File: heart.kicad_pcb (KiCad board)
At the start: 2 copper layers, 94 x 78.7 mm, 20 parts, among them J1 Positive, J2 Negative, J3 Conn_01x19_Female, J4 Conn_01x19_Female, P1 USB_C_Plug_USB2.0, SW1 SW_DIP_x01, U1 BMD101, U2 TP4054, U3 RS3236, U5 RS8051

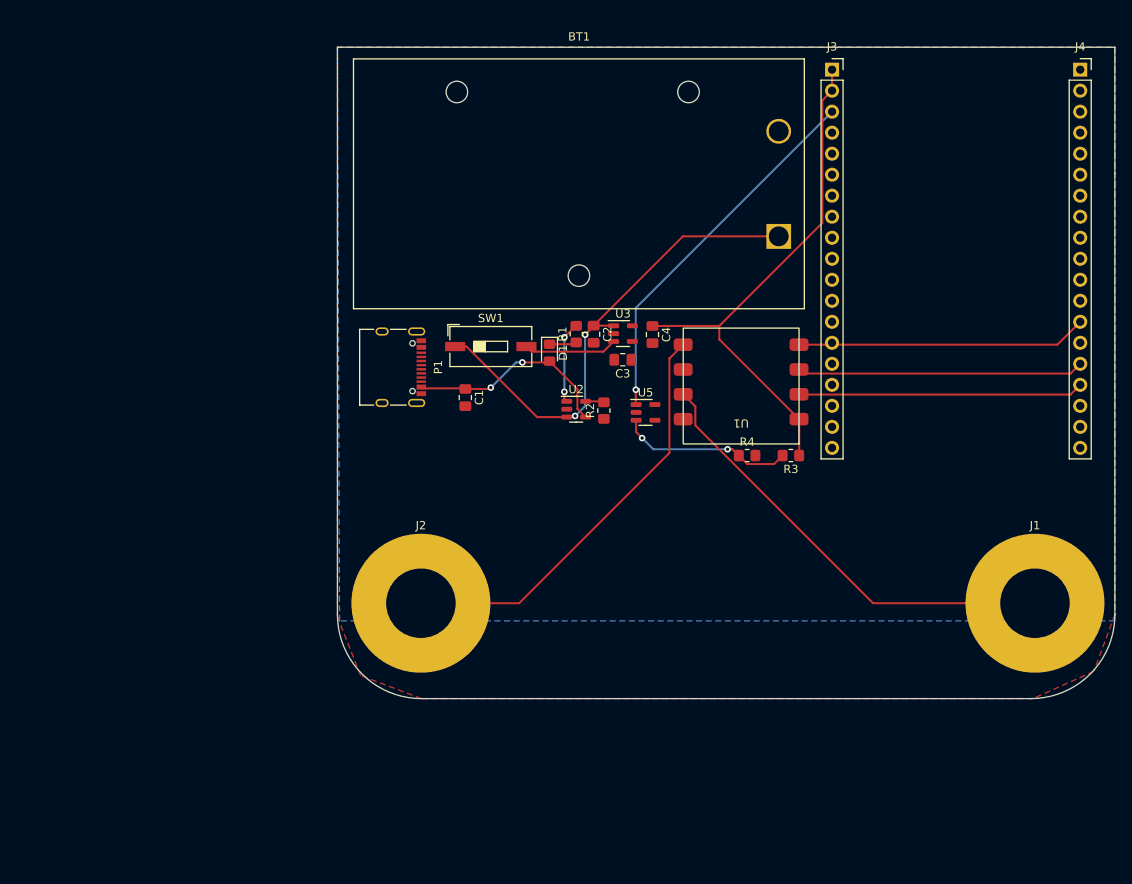
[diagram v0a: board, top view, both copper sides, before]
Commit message: 最终投板
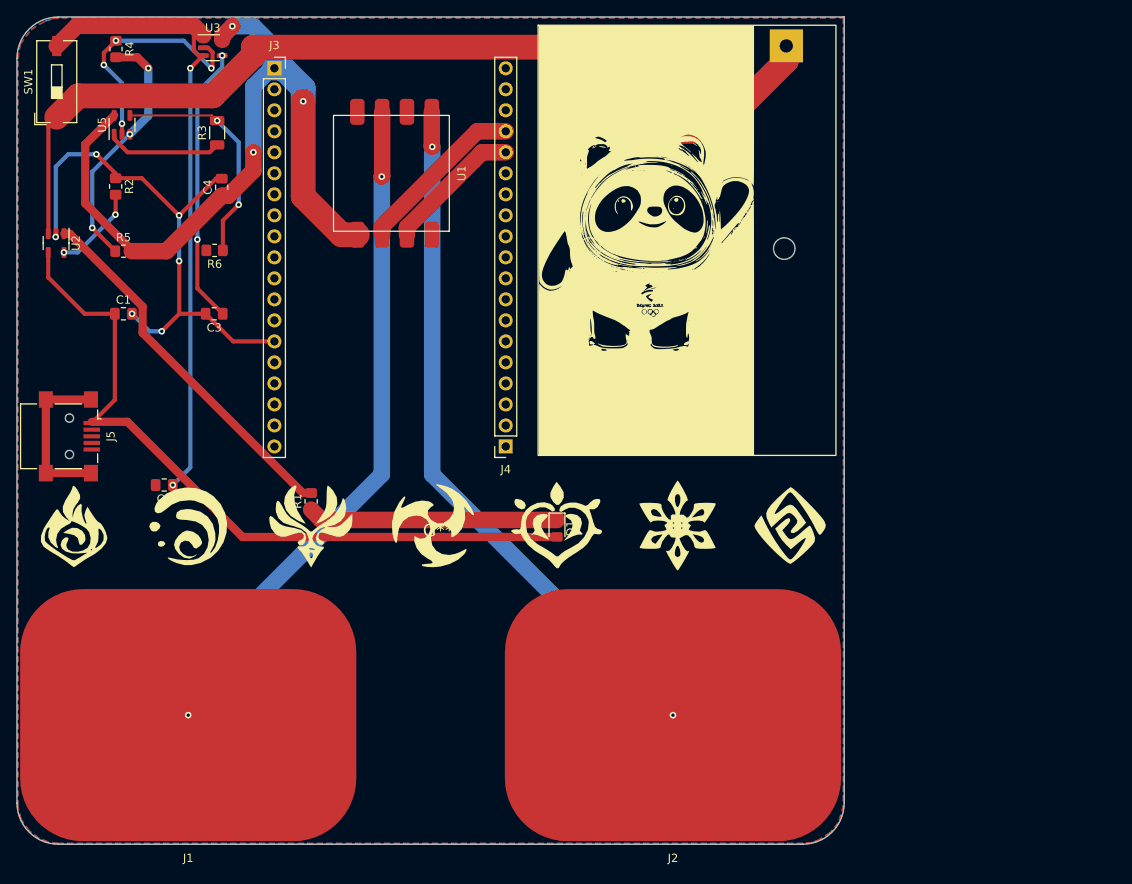
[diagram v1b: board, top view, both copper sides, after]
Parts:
- removed P1: USB_C_Plug_USB2.0, Connector_USB:USB_C_Receptacle_XKB_U262-16XN-4BVC11
- added G***: LOGO, My_Print:ys, F.Cu at (91.4, 132.1)
- added G***: LOGO, My_Print:bdd, F.Cu at (116.1, 97.0)
- added G***: LOGO, My_Print:SL_100x100, B.Cu at (89.8, 120.2)
- added J5: USB_B_Mini, Connector_USB:USB_Mini-B_Lumberg_2486_01_Horizontal, F.Cu at (46.3, 120.7)
- added R5: 30 k, Resistor_SMD:R_0805_2012Metric_Pad1.20x1.40mm_HandSolder, F.Cu at (52.9, 98.3)
- added R6: 10 k, Resistor_SMD:R_0805_2012Metric_Pad1.20x1.40mm_HandSolder, F.Cu at (63.9, 98.2)
- BT1: footprint Battery:BatteryHolder_Eagle_12BH611-GR -> My_Print:battary
- J1, J2: footprint MountingHole:MountingHole_8.4mm_M8_Pad -> My_Print:Square_Pad_40mm*30mm
- R3: footprint Resistor_SMD:R_0805_2012Metric_Pad1.20x1.40mm_HandSolder -> Resistor_SMD:R_1206_3216Metric
- R4: value 1K -> 10 k
- U1: footprint Package_TO_SOT_SMD:BMD101 -> My_Print:BMD101
- moved J1 107.0 mm to (60.7, 172.2)
- moved R4 90.8 mm to (52.0, 73.9), turned to -90 degrees
- moved J4 83.1 mm to (99.1, 121.9), turned to 180 degrees
- moved R3 79.6 mm to (64.2, 84.0), turned to 90 degrees
- moved U5 72.2 mm to (52.7, 83.0), turned to 90 degrees
- moved J3 67.4 mm to (71.1, 76.2)
- moved U2 66.0 mm to (44.7, 97.3), turned to -90 degrees
- moved R2 64.9 mm to (51.9, 90.5), turned to -90 degrees
- moved SW1 61.5 mm to (44.8, 77.8), turned to 90 degrees
- moved U3 60.4 mm to (63.7, 73.7)
- moved C4 55.0 mm to (64.8, 90.6), turned to 90 degrees
- moved C2 55.0 mm to (57.8, 126.6), turned to 180 degrees
- moved C3 49.7 mm to (63.8, 105.9)
- moved J2 43.7 mm to (119.3, 172.2)
- moved C1 42.6 mm to (52.9, 105.9), turned to 0 degrees
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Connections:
- C2 pad 1: /BT+ -> Net-(C2-Pad1)
- J3 pad 2: /VCC -> unconnected-(J3-Pad2)
- R3 pad 1: /VCC -> Net-(R3-Pad1)
- R3 pad 2: /Temp -> Net-(R3-Pad2)
- R4 pad 1: /Temp -> GNDREF
- R4 pad 2: GNDREF -> Net-(R4-Pad2)
- SW1 pad 2: Net-(SW1-Pad2) -> Net-(C2-Pad1)
- U3 pad 1: /BT+ -> Net-(C2-Pad1)
- U3 pad 3: Net-(SW1-Pad2) -> Net-(C2-Pad1)
- U5 pad 1: /ADC -> Net-(R3-Pad1)
- U5 pad 2: unconnected-(U5-Pad2) -> GNDREF
- U5 pad 3: /Temp -> Net-(R4-Pad2)
- U5 pad 4: unconnected-(U5-Pad4) -> Net-(R3-Pad2)
- U5 pad 5: unconnected-(U5-Pad5) -> /VCC
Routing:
- net Net-(C2-Pad1): track 0.00 -> 77.1 mm, vias 0 -> 2
- net Net-(C1-Pad1): track 25.5 -> 89.3 mm, vias 2 -> 0
- net GNDREF: track 35.1 -> 95.7 mm, vias 0 -> 10
- net /BT+: track 59.2 -> 116.3 mm, vias 2 -> 0
- net /ADC: track 45.2 -> 0.00 mm, vias 1 -> 0
- net Net-(R1-Pad2): track 9.88 -> 44.7 mm, vias 2 -> 0
- net Net-(C3-Pad1): track 0.00 -> 33.7 mm, vias 0 -> 2
- net Net-(J2-Pad1): track 51.3 -> 85.0 mm, vias 0 -> 2
- net Net-(R4-Pad2): track 0.00 -> 30.5 mm, vias 0 -> 3
- net Net-(R3-Pad2): track 0.00 -> 28.4 mm, vias 0 -> 2
- net Net-(J1-Pad1): track 54.3 -> 82.6 mm, vias 0 -> 2
- net Net-(D1-Pad1): track 3.32 -> 30.2 mm
- net /VCC: track 64.4 -> 89.4 mm, vias 0 -> 3
- net /Temp: track 21.2 -> 0.00 mm, vias 2 -> 0
- net unconnected-(J5-Pad6): track 0.00 -> 19.8 mm
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- added copper zone on B.Cu, net GNDREF
- removed copper zone on B.Cu, net /VCC
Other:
- board size 94 x 78.7 mm -> 100 x 100 mm
